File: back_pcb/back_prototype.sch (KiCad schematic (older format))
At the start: 27 parts, among them U1 Pi0Top

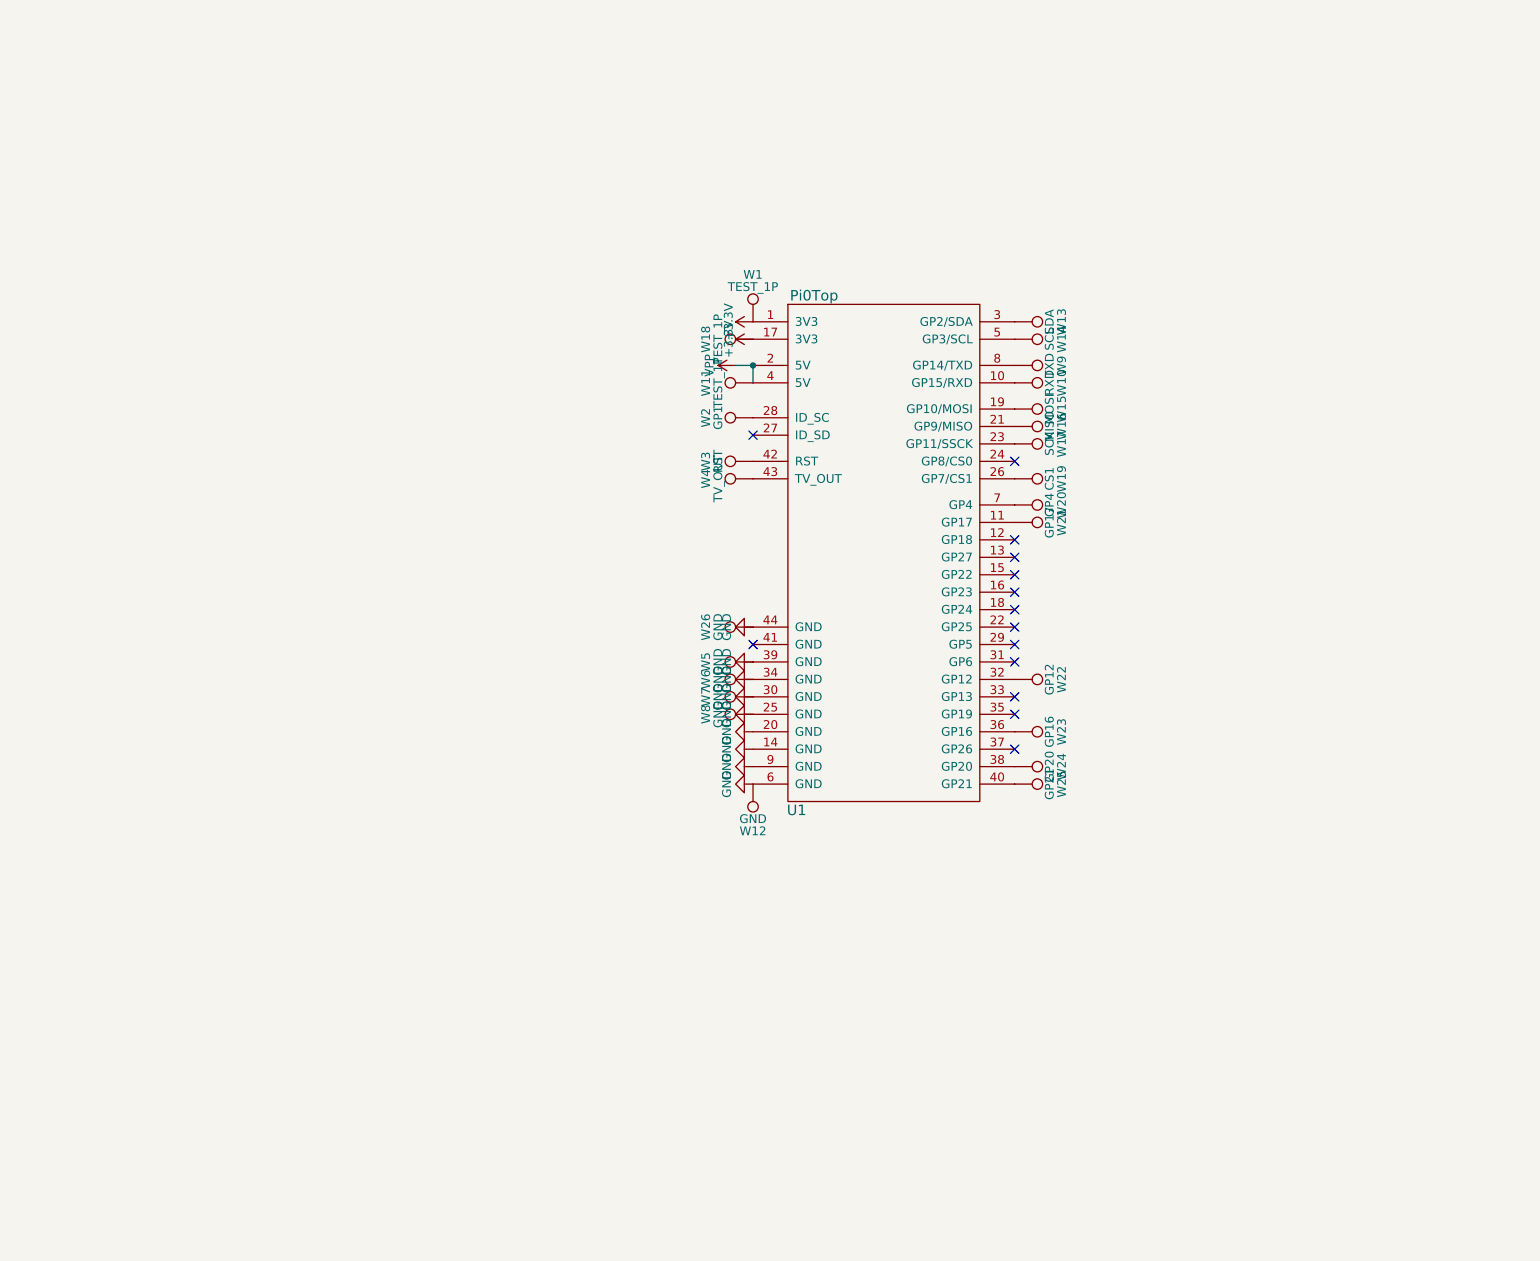
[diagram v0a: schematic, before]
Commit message: Started new back PCB
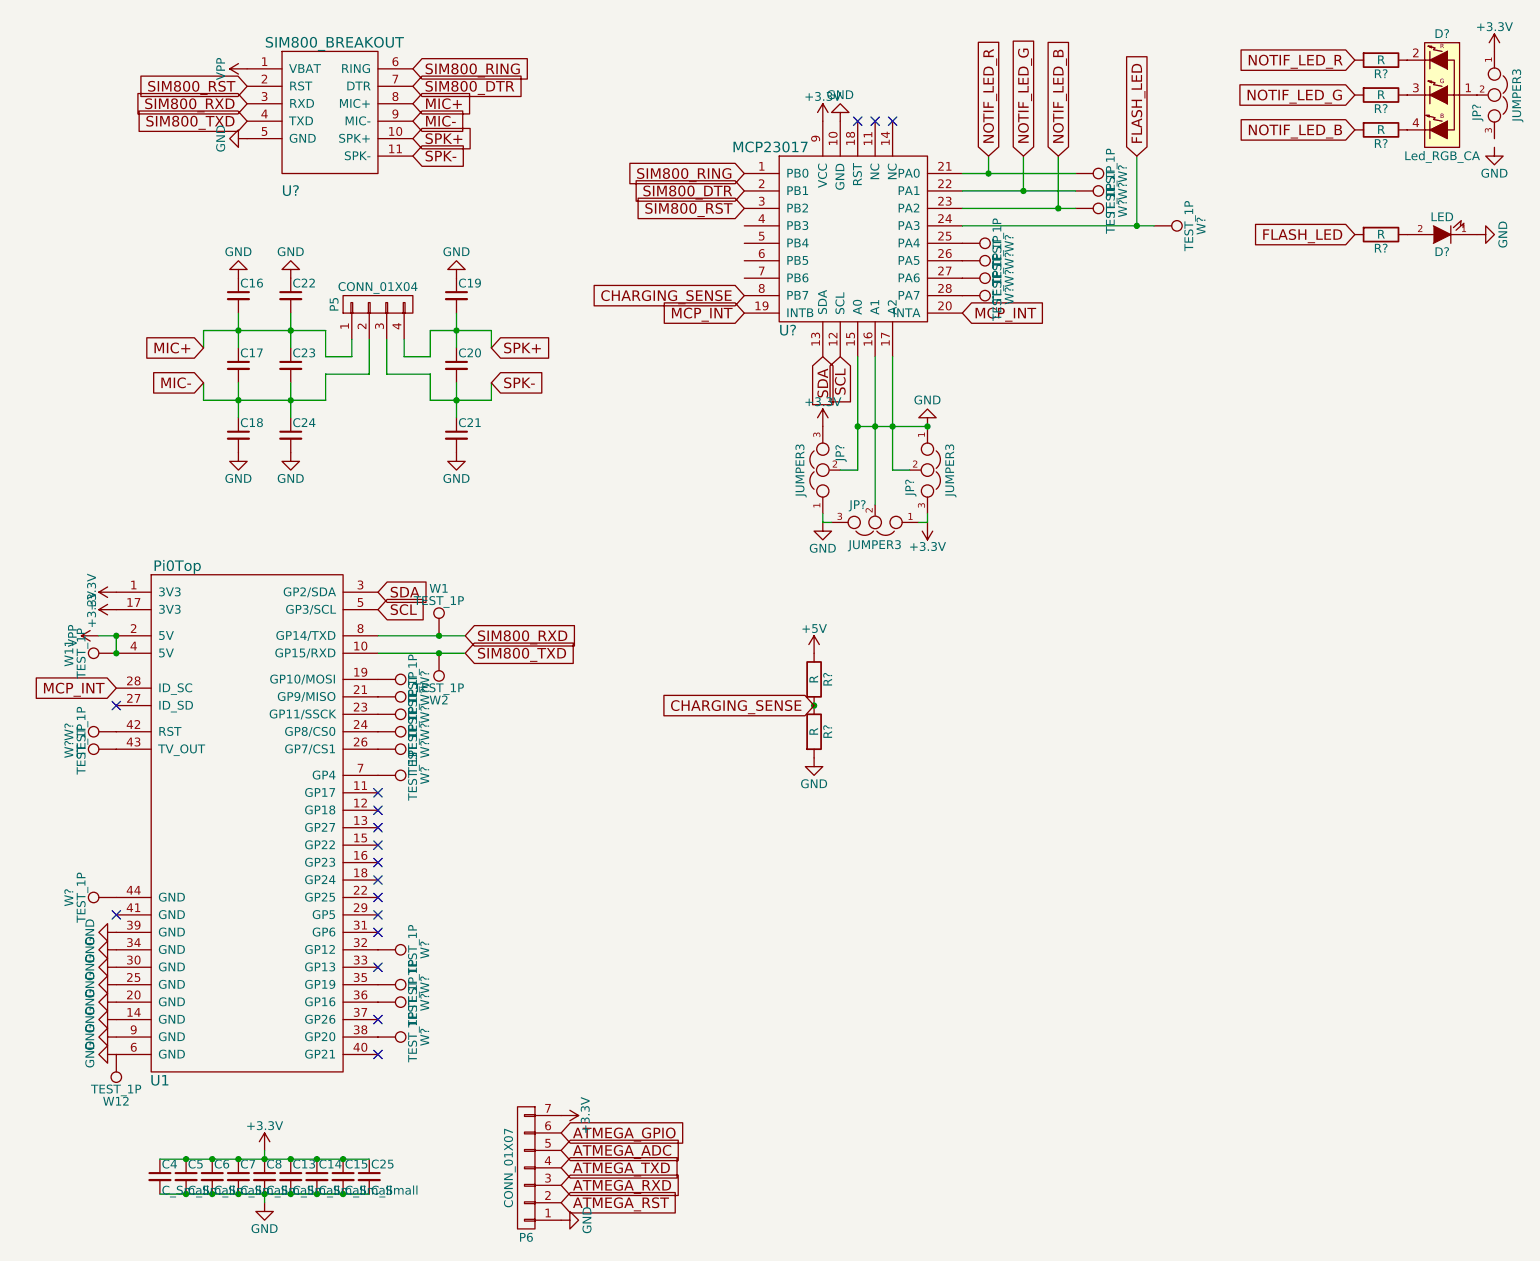
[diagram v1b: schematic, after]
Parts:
- removed W10: RXD, Measurement_Points:Measurement_Point_Square-SMD-Pad_Small, symbol TEST_1P
- removed W13: SDA, Measurement_Points:Measurement_Point_Square-SMD-Pad_Small, symbol TEST_1P
- removed W14: SCL, Measurement_Points:Measurement_Point_Square-SMD-Pad_Small, symbol TEST_1P
- removed W15: MOSI, Measurement_Points:Measurement_Point_Square-SMD-Pad_Small, symbol TEST_1P
- removed W16: MISO, Measurement_Points:Measurement_Point_Square-SMD-Pad_Small, symbol TEST_1P
- removed W17: SCK, Measurement_Points:Measurement_Point_Square-SMD-Pad_Small, symbol TEST_1P
- removed W18: TEST_1P, Measurement_Points:Measurement_Point_Square-SMD-Pad_Small, symbol TEST_1P
- removed W19: CS1, Measurement_Points:Measurement_Point_Square-SMD-Pad_Small, symbol TEST_1P
- removed W20: GP4, Measurement_Points:Measurement_Point_Square-SMD-Pad_Small, symbol TEST_1P
- removed W21: GP17, Measurement_Points:Measurement_Point_Square-SMD-Pad_Small, symbol TEST_1P
- removed W22: GP12, Measurement_Points:Measurement_Point_Square-SMD-Pad_Small, symbol TEST_1P
- removed W23: GP16, Measurement_Points:Measurement_Point_Square-SMD-Pad_Small, symbol TEST_1P
- removed W24: GP20, Measurement_Points:Measurement_Point_Square-SMD-Pad_Small, symbol TEST_1P
- removed W25: GP21, Measurement_Points:Measurement_Point_Square-SMD-Pad_Small, symbol TEST_1P
- removed W26, W5, W6, W7, W8: GND, Measurement_Points:Measurement_Point_Square-SMD-Pad_Small, symbol TEST_1P
- removed W3: RST, Measurement_Points:Measurement_Point_Square-SMD-Pad_Small, symbol TEST_1P
- removed W4: TV_OUT, Measurement_Points:Measurement_Point_Square-SMD-Pad_Small, symbol TEST_1P
- removed W9: TXD, Measurement_Points:Measurement_Point_Square-SMD-Pad_Small, symbol TEST_1P
- added C13, C14, C15, C25, C4, C5, C6, C7, C8: C_Small, Capacitors_SMD:C_0805, symbol C_Small
- added C16, C17, C18, C19, C20, C21, C22, C23, C24: C_Small, Capacitors_SMD:C_0603, symbol C_Small
- added D?: Led_RGB_CA, symbol Led_RGB_CA
- added D?: LED, symbol LED
- added JP? (x4): JUMPER3, symbol JUMPER3
- added P5: CONN_01X04, Pin_Headers:Pin_Header_Straight_1x04_Pitch2.54mm, symbol CONN_01X04
- added P6: CONN_01X07, Pin_Headers:Pin_Header_Straight_1x07_Pitch2.54mm, symbol CONN_01X07
- added R? (x6): R, symbol R
- added U?: SIM800_BREAKOUT, symbol SIM800_BREAKOUT
- added U?: MCP23017, symbol MCP23017
- added W? (x21): TEST_1P, Measurement_Points:Measurement_Point_Square-SMD-Pad_Small, symbol TEST_1P
- U1: footprint Pi0Top:Pi0Top -> common-footprints:pi0outline
- W12: value GND -> TEST_1P
- W2: value GP1 -> TEST_1P
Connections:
- net +3V3: now also C13.1, C14.1, C15.1, C25.1, C4.1, C5.1, C6.1, C7.1, C8.1, JP?.1, JP?.1, JP?.3, JP?.3, P6.7 (P7), U?.9 (VCC); no longer W1.1
- net GND: now also C13.2, C14.2, C15.2, C16.1, C18.2, C19.1, C21.2, C22.1, C24.2, C25.2, C4.2, C5.2, C6.2, C7.2, C8.2, D?.1 (K), JP?.1, JP?.1, JP?.2, JP?.2, JP?.2, JP?.3, P6.1 (P1), R?.2, U?.10 (GND), U?.15 (A0), U?.16 (A1), U?.17 (A2), U?.5 (GND); no longer U1.44 (GND)
- net VPP: now also U?.1 (VBAT)
- net SIM800_TXD: now reaches U1.10 (GP15/RXD)
- net SIM800_TXD: now also W2.1, U?.4 (TXD)
- net at U1.19 (GP10/MOSI): now also W?.1
- net at U1.21 (GP9/MISO): now also W?.1
- net at U1.23 (GP11/SSCK): now also W?.1
- net at U1.24 (GP8/CS0): now also W?.1
- net at U1.26 (GP7/CS1): now also W?.1
- net MCP_INT: now reaches U1.28 (ID_SC)
- net MCP_INT: now also U?.19 (INTB), U?.20 (INTA); no longer W2.1
- net SDA: now reaches U1.3 (GP2/SDA)
- net SDA: now also U?.13 (SDA)
- net at U1.32 (GP12): now also W?.1
- net at U1.35 (GP19): now also W?.1
- net at U1.36 (GP16): now also W?.1
- net at U1.38 (GP20): now also W?.1
- net at U1.42 (RST): now also W?.1
- net at U1.43 (TV_OUT): now also W?.1
- net SCL: now reaches U1.5 (GP3/SCL)
- net SCL: now also U?.12 (SCL)
- net at U1.7 (GP4): now also W?.1
- net SIM800_RXD: now reaches U1.8 (GP14/TXD)
- net SIM800_RXD: now also W1.1, U?.3 (RXD)
- new net: U1.44 (GND), W?.1
- new net: U?.25 (PA4), W?.1
- new net: U?.26 (PA5), W?.1
- new net: U?.27 (PA6), W?.1
- new net: U?.28 (PA7), W?.1
- new net: D?.1, JP?.2
- new net: D?.2 (R), R?.1
- new net: D?.3 (G), R?.1
- new net: D?.4 (B), R?.1
- new net: D?.2 (A), R?.1
- new net +5V: R?.1
- new net ATMEGA_ADC: P6.5 (P5)
- new net ATMEGA_GPIO: P6.6 (P6)
- new net ATMEGA_RST: P6.2 (P2)
- new net ATMEGA_RXD: P6.3 (P3)
- new net ATMEGA_TXD: P6.4 (P4)
- new net CHARGING_SENSE: R?.1, R?.2, U?.8 (PB7)
- new net FLASH_LED: R?.2, U?.24 (PA3), W?.1
- new net MIC+: C16.2, C17.1, C22.2, C23.1, P5.1 (P1), U?.8 (MIC+)
- new net MIC-: C17.2, C18.1, C23.2, C24.1, P5.2 (P2), U?.9 (MIC-)
- new net NOTIF_LED_B: R?.2, U?.23 (PA2), W?.1
- new net NOTIF_LED_G: R?.2, U?.22 (PA1), W?.1
- new net NOTIF_LED_R: R?.2, U?.21 (PA0), W?.1
- new net SIM800_DTR: U?.2 (PB1), U?.7 (DTR)
- new net SIM800_RING: U?.1 (PB0), U?.6 (RING)
- new net SIM800_RST: U?.2 (RST), U?.3 (PB2)
- new net SPK+: C19.2, C20.1, P5.4 (P4), U?.10 (SPK+)
- new net SPK-: C20.2, C21.1, P5.3 (P3), U?.11 (SPK-)
- no-connect marks 14 -> 17
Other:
- moved on the sheet: U1, W11, W12
